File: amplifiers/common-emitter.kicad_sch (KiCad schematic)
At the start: 21 parts, among them Q1 PNP, Q2 Q_NPN

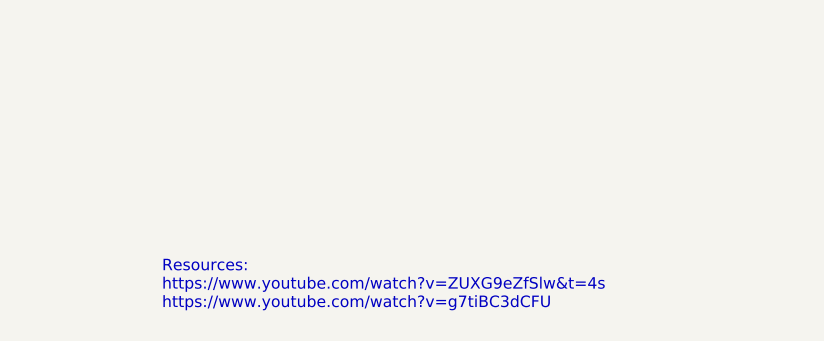
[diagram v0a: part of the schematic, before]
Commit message: wip save
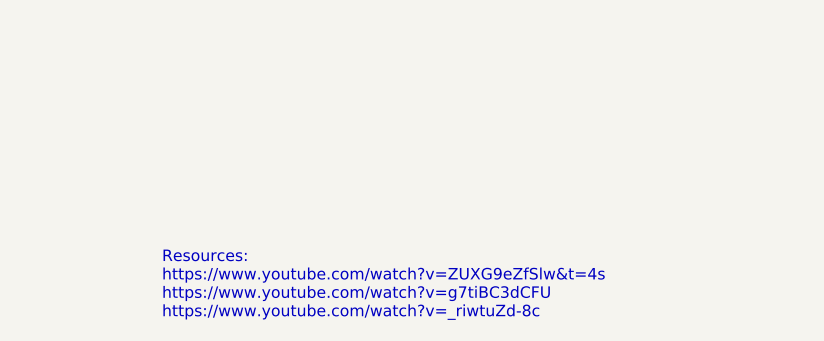
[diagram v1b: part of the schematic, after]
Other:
- note added: "Resources: https://www.youtube.com/watch?v=ZUXG9eZfSlw&t=4s https://www.youtube.com/watch?v=g7tiBC3dCFU https://www.youtube.com/watch?v=_riwtuZd-8c"
- note removed: "Resources: https://www.youtube.com/watch?v=ZUXG9eZfSlw&t=4s https://www.youtube.com/watch?v=g7tiBC3dCFU"
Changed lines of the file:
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@@
 		)
 	)
-	(text "Resources:\nhttps://www.youtube.com/watch?v=ZUXG9eZfSlw&t=4s\nhttps://www.youtube.com/watch?v=g7tiBC3dCFU"
+	(text "Resources:\nhttps://www.youtube.com/watch?v=ZUXG9eZfSlw&t=4s\nhttps://www.youtube.com/watch?v=g7tiBC3dCFU\nhttps://www.youtube.com/watch?v=_riwtuZd-8c"
 		(exclude_from_sim no)
 		(at 223.774 155.956 0)
